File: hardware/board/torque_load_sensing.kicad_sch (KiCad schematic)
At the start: 22 parts, among them J3 Conn_01x05_Female, U7 AD8226, U8 ADS7049

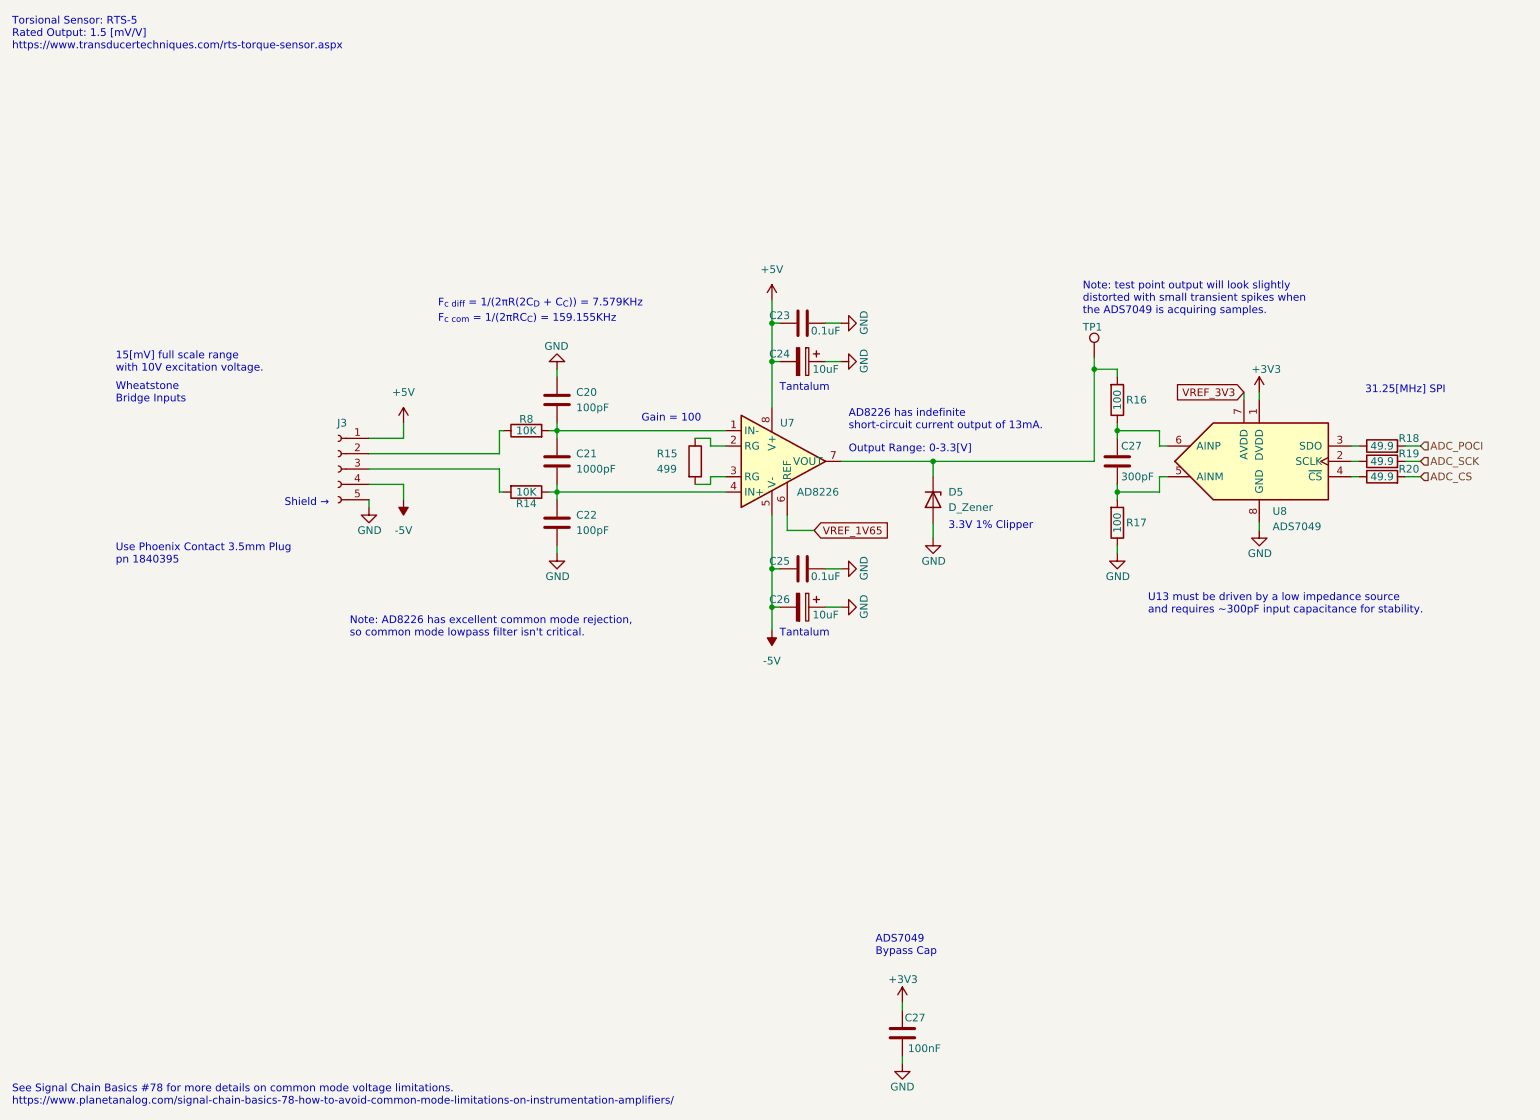
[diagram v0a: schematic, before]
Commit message: update schematic; continue pcb draft
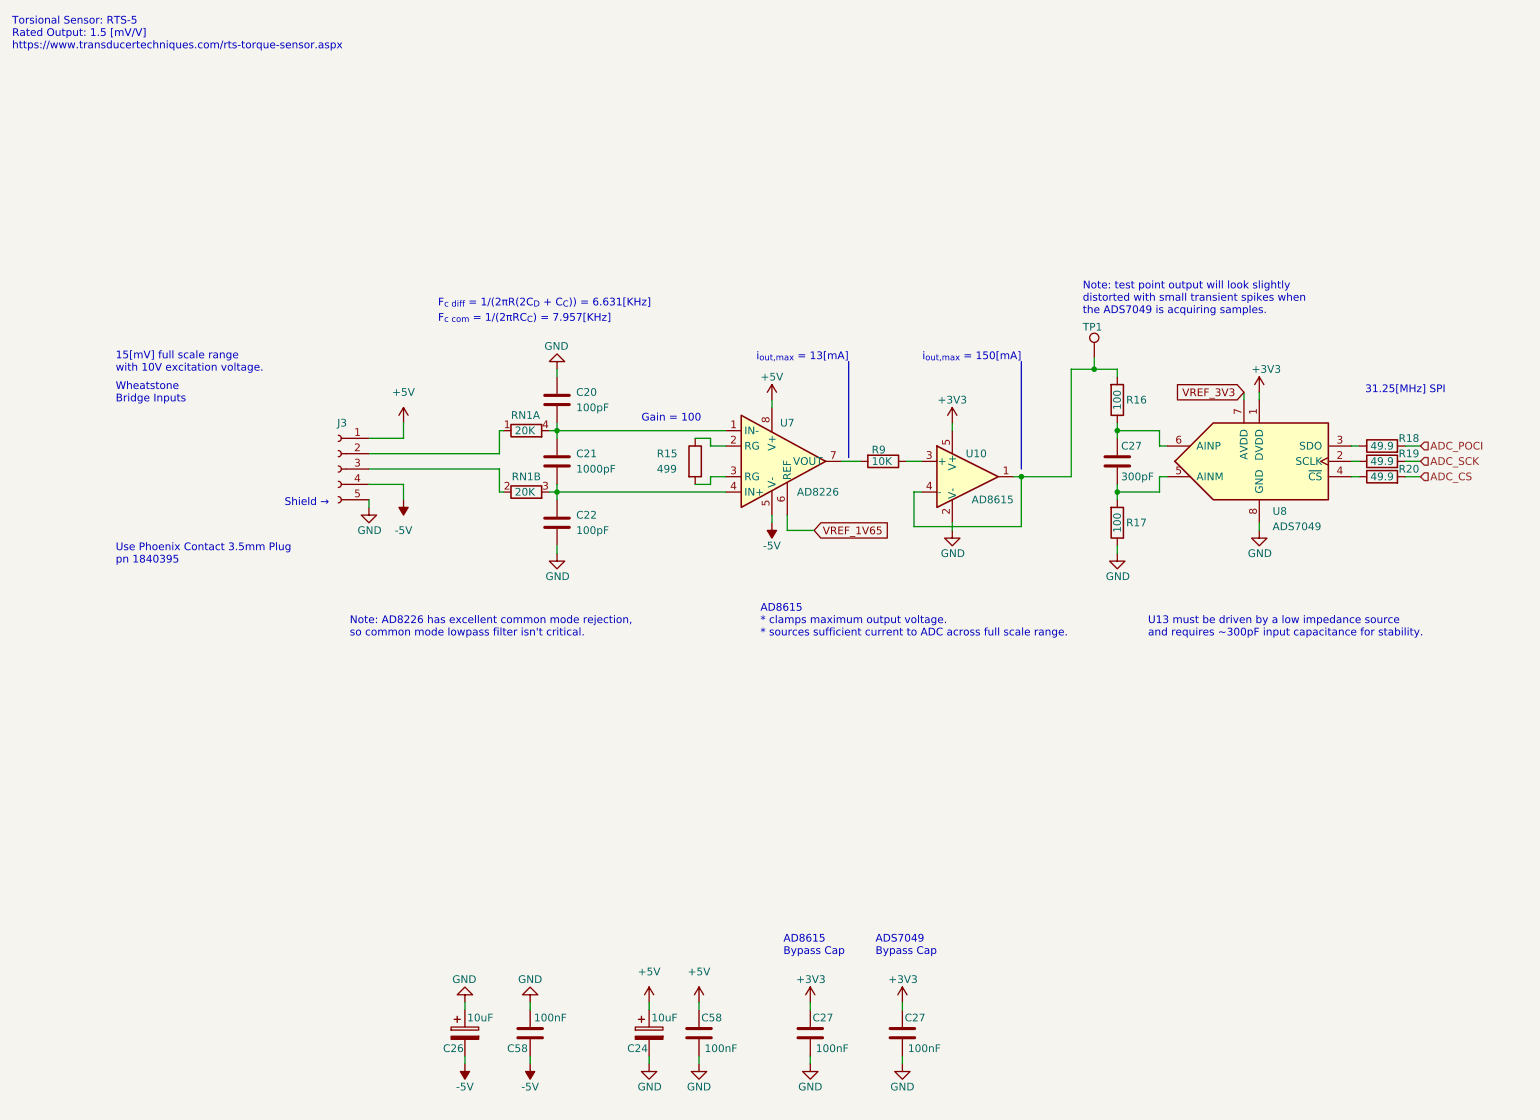
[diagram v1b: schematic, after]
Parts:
- removed C23, C25: 0.1uF, symbol Device:C
- removed D5: D_Zener, Diode_SMD:D_SOD-123F, symbol Device:D_Zener
- removed R14, R8: 10K, Resistor_SMD:R_0402_1005Metric, symbol Device:R
- added C27, C58 (x2): 100nF, Capacitor_SMD:C_0402_1005Metric, symbol Device:C
- added R9: 10K, Resistor_SMD:R_0402_1005Metric, symbol Device:R
- added RN1: 20K, Resistor_SMD:R_Array_Convex_2x0606, symbol Device:R_Pack02_Split
- added U10: AD8615, Package_TO_SOT_SMD:TSOT-23-5, symbol kicad_component_library:AD8615
- C20, C22: footprint (none) -> Capacitor_SMD:C_0402_1005Metric; Link https://www.digikey.com/en/products/detail/murata-electroni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 -> https://www.digikey.com/en/products/detail/kyocera-avx/KGM0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; Manufacturer Murata Electronics -> KYOCERA AVX; Manufacturer Number GCM1555C1H101FA16D -> KGM05ACG1H101FH
- C21: footprint (none) -> Capacitor_SMD:C_0402_1005Metric; Link https://www.digikey.com/en/products/detail/murata-electronics/GCM1555C1H101FA16D/6605978 -> https://www.digikey.com/en/products/detail/murata-electronics/GRM1555C1H102JA01D/702509; Manufacturer Number GCM1555C1H101FA16D -> GRM1555C1H102JA01D
- C24, C26: Alternate GRM21BR61H106KE43L -> (none); Link https://www.digikey.com/en/products/detail/murata-electroni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 -> https://www.digikey.com/en/products/detail/kemet/T529P106M0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; Manufacturer Murata Electronics -> Kemet; Manufacturer Number GRM21BR61H106KE43L -> T529P106M010AAE200; Notes (none) -> polarized, anode band; Rated Voltage 50V -> 10V; Temperature Coefficient X5R -> (none); Tolerance 10% -> 20%
- R15: footprint Resistor_SMD:R_0603_1608Metric -> Resistor_SMD:R_0603_1608Metric_Pad0.98x0.95mm_HandSolder
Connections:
- net +3V3: now also C27.2, U10.5 (V+)
- net +5V: now also C24.1, C58.2; no longer C24.2
- net -5V: now also C58.2
- net GND: now also C24.2, C27.1, C58.1, C58.1, U10.2 (V-); no longer C24.1
- net at C20.2, C21.1, U7.1 (IN-): now also RN1.4 (R1.2)
- net at C21.2, C22.1, U7.4 (IN+): now also RN1.3 (R2.2)
- net at R16.2, TP1.1: now also U10.1, U10.4 (-); no longer U7.7 (VOUT)
- net at J3.2 (Pin_2): now also RN1.1 (R1.1)
- net at J3.3 (Pin_3): now also RN1.2 (R2.1)
- new net: R9.2, U7.7 (VOUT)
- new net: R9.1, U10.3 (+)
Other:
- note added: "AD8615 * clamps maximum output voltage. * sources sufficient current to ADC across full scale range."
- note added: "AD8615 Bypass Cap"
- note added: "F_{c com} = 1/(2πRC_{C}) = 7.957[KHz]"
- note added: "F_{c diff} = 1/(2πR(2C_{D} + C_{C})) = 6.631[KHz]"
- note added: "i_{out,max} = 13[mA]"
- note added: "i_{out,max} = 150[mA]"
- note removed: "3.3V 1% Clipper"
- note removed: "AD8226 has indefinite short-circuit current output of 13mA."
- note removed: "F_{c com} = 1/(2πRC_{C}) = 159.155KHz"
- note removed: "F_{c diff} = 1/(2πR(2C_{D} + C_{C})) = 7.579KHz"
- note removed: "Output Range: 0-3.3[V]"
- note removed: "See Signal Chain Basics #78 for more details on common mode voltage limitations. https://www.planetanalog.com/signal-chain-basics-78-how-to-avoid-common-mode-limitations-on-instrumentation-amplifiers/"
- note removed: "Tantalum"
- moved on the sheet: C26
